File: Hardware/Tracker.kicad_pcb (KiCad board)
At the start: 2 copper layers, 233.7 x 114.2 mm, 58 parts, among them J1 Battery, J10 132134, J11 SPI_Programming, J2 Motor, J3 Wind, J4 RX, J5 TX, J6 GND, J7 GND, J8 GND, J9 Haeder_LED, U1 L7805, U2 ATmega328P-P, U3 LM317_TO-220, U4 L298N, U5 74HC123, U6 LM358, U7 GK9501, Y1 16MHz

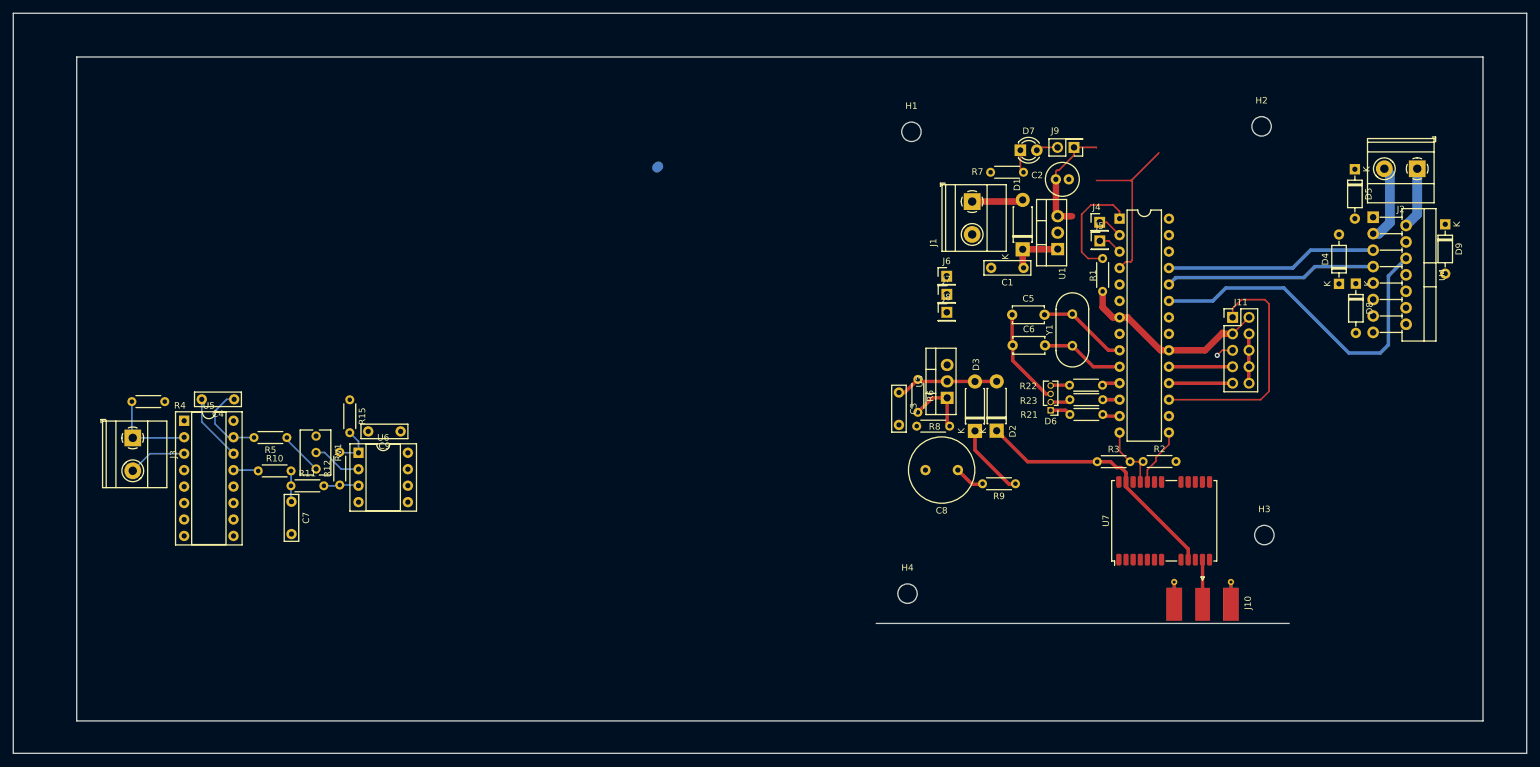
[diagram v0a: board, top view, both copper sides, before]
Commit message: Update of PCB
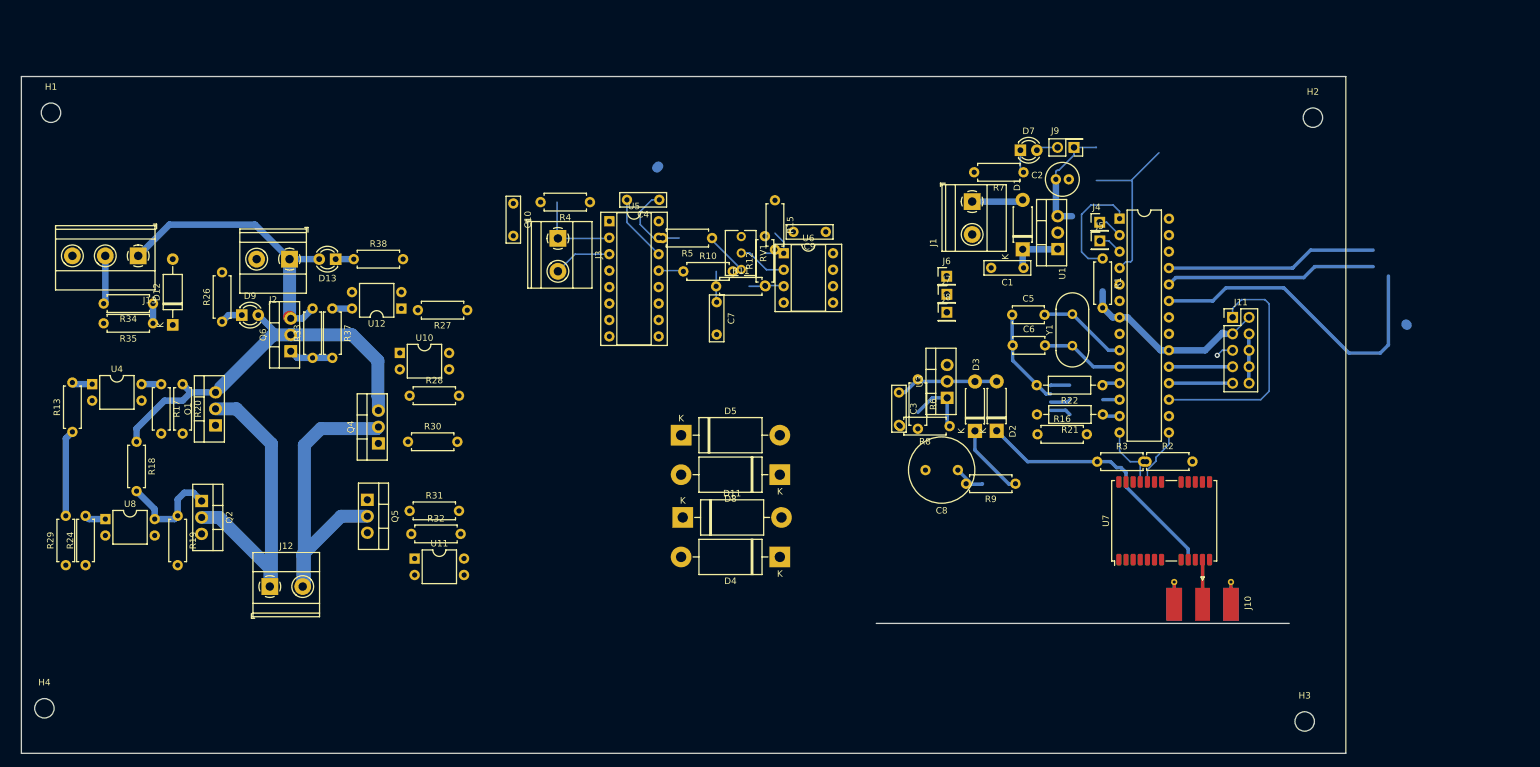
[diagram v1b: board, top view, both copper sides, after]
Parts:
- removed D6: LED_RBKG, Connector_PinHeader_1.27mm:PinHeader_1x04_P1.27mm_Vertical
- removed R23: 270, Resistor_THT:R_Axial_DIN0204_L3.6mm_D1.6mm_P5.08mm_Horizontal
- added C10: 100nF, Capacitor_THT:C_Rect_L7.0mm_W2.0mm_P5.00mm, F.Cu at (82.3, 68.1)
- added D11: 1N5406, Diode_THT:D_DO-201AD_P15.24mm_Horizontal, F.Cu at (108.5, 116.6)
- added D12: 3.3V, Diode_THT:D_A-405_P10.16mm_Horizontal, F.Cu at (29.7, 86.9)
- added D13: LED, LED_THT:LED_D3.0mm, F.Cu at (54.9, 76.7)
- added J12: Sortie Moteur, TerminalBlock_Phoenix:TerminalBlock_Phoenix_MKDS-1,5-2-5.08_1x02_P5.08mm_Horizontal, F.Cu at (44.7, 127.3)
- added J13: Position_Potentiometer, TerminalBlock_Phoenix:TerminalBlock_Phoenix_MKDS-1,5-3-5.08_1x03_P5.08mm_Horizontal, F.Cu at (24.4, 76.2)
- added Q1: IRF4905, Package_TO_SOT_THT:TO-220-3_Vertical, F.Cu at (36.3, 102.4)
- added Q2: IRF520, Package_TO_SOT_THT:TO-220-3_Vertical, F.Cu at (34.2, 114.0)
- added Q4: IRF4905, Package_TO_SOT_THT:TO-220-3_Vertical, F.Cu at (61.5, 105.2)
- added Q5: IRF520, Package_TO_SOT_THT:TO-220-3_Vertical, F.Cu at (59.8, 113.9)
- added Q6: IRF4905, Package_TO_SOT_THT:TO-220-3_Vertical, F.Cu at (47.9, 90.9)
- added R13: 470, Resistor_THT:R_Axial_DIN0207_L6.3mm_D2.5mm_P7.62mm_Horizontal, F.Cu at (14.2, 103.4)
- added R16: 470, Resistor_THT:R_Axial_DIN0207_L6.3mm_D2.5mm_P7.62mm_Horizontal, F.Cu at (163.2, 103.8)
- added R17: 2.2K, Resistor_THT:R_Axial_DIN0207_L6.3mm_D2.5mm_P7.62mm_Horizontal, F.Cu at (27.9, 96.0)
- added R18: 1K, Resistor_THT:R_Axial_DIN0207_L6.3mm_D2.5mm_P7.62mm_Horizontal, F.Cu at (24.1, 104.9)
- added R19: 100k, Resistor_THT:R_Axial_DIN0207_L6.3mm_D2.5mm_P7.62mm_Horizontal, F.Cu at (30.5, 116.3)
- added R20: 1K, Resistor_THT:R_Axial_DIN0207_L6.3mm_D2.5mm_P7.62mm_Horizontal, F.Cu at (31.2, 96.0)
- added R24: 470, Resistor_THT:R_Axial_DIN0207_L6.3mm_D2.5mm_P7.62mm_Horizontal, F.Cu at (16.3, 124.0)
- added R26: 3.3K, Resistor_THT:R_Axial_DIN0207_L6.3mm_D2.5mm_P7.62mm_Horizontal, F.Cu at (37.3, 86.4)
- added R27: 470, Resistor_THT:R_Axial_DIN0207_L6.3mm_D2.5mm_P7.62mm_Horizontal, F.Cu at (75.2, 84.6)
- added R28: 1K, Resistor_THT:R_Axial_DIN0207_L6.3mm_D2.5mm_P7.62mm_Horizontal, F.Cu at (66.3, 97.8)
- added R29: 470, Resistor_THT:R_Axial_DIN0207_L6.3mm_D2.5mm_P7.62mm_Horizontal, F.Cu at (13.2, 124.0)
- added R30: 2.2K, Resistor_THT:R_Axial_DIN0207_L6.3mm_D2.5mm_P7.62mm_Horizontal, F.Cu at (66.0, 104.9)
- added R31: 1K, Resistor_THT:R_Axial_DIN0207_L6.3mm_D2.5mm_P7.62mm_Horizontal, F.Cu at (66.3, 115.6)
- added R32: 100k, Resistor_THT:R_Axial_DIN0207_L6.3mm_D2.5mm_P7.62mm_Horizontal, F.Cu at (66.5, 119.1)
- added R33: 1k, Resistor_THT:R_Axial_DIN0207_L6.3mm_D2.5mm_P7.62mm_Horizontal, F.Cu at (51.3, 91.9)
- added R34: 2.7K, Resistor_THT:R_Axial_DIN0207_L6.3mm_D2.5mm_P7.62mm_Horizontal, F.Cu at (26.7, 83.6)
- added R35: 1K, Resistor_THT:R_Axial_DIN0207_L6.3mm_D2.5mm_P7.62mm_Horizontal, F.Cu at (26.7, 86.6)
- added R37: 2.2K, Resistor_THT:R_Axial_DIN0207_L6.3mm_D2.5mm_P7.62mm_Horizontal, F.Cu at (54.4, 84.3)
- added R38: 3.3K, Resistor_THT:R_Axial_DIN0207_L6.3mm_D2.5mm_P7.62mm_Horizontal, F.Cu at (57.7, 76.7)
- added U10: PC817, Package_DIP:DIP-4_W7.62mm, F.Cu at (64.8, 91.2)
- added U11: PC817, Package_DIP:DIP-4_W7.62mm, F.Cu at (67.1, 122.9)
- added U12: PC817, Package_DIP:DIP-4_W7.62mm, F.Cu at (65.0, 84.3)
- added U8: PC817, Package_DIP:DIP-4_W7.62mm, F.Cu at (19.3, 116.8)
- D2, D3: value D -> 1N4818
- D4, D5, D8: value 1N4148 -> 1N5406; footprint Diode_THT:D_DO-35_SOD27_P7.62mm_Horizontal -> Diode_THT:D_DO-201AD_P15.24mm_Horizontal
- D9: value 1N4148 -> LED; footprint Diode_THT:D_DO-35_SOD27_P7.62mm_Horizontal -> LED_THT:LED_D3.0mm
- J2: value Motor -> +24V
- R1, R10, R11, R12, R15, R2, R3, R4, R5, R6, R7, R8, R9: footprint Resistor_THT:R_Axial_DIN0204_L3.6mm_D1.6mm_P5.08mm_Horizontal -> Resistor_THT:R_Axial_DIN0207_L6.3mm_D2.5mm_P7.62mm_Horizontal
- R21, R22: footprint Resistor_THT:R_Axial_DIN0204_L3.6mm_D1.6mm_P5.08mm_Horizontal -> Resistor_THT:R_Axial_DIN0207_L6.3mm_D2.5mm_P10.16mm_Horizontal
- U4: value L298N -> PC817; footprint Package_TO_SOT_THT:TO-220-15_P2.54x2.54mm_StaggerOdd_Lead4.58mm_Vertical -> Package_DIP:DIP-4_W7.62mm
- moved U4 199.4 mm to (17.3, 96.0), turned to 0 degrees
- moved D9 186.3 mm to (40.4, 85.3), turned to 0 degrees
- moved J2 174.7 mm to (47.8, 76.7)
- moved H4 134.4 mm to (9.91, 146.1)
- moved H1 132.9 mm to (10.9, 54.1)
- moved D5 111.8 mm to (108.2, 103.9), turned to 0 degrees
- moved D4 96.1 mm to (123.4, 122.7), turned to 180 degrees
- moved D8 93.7 mm to (123.4, 110.0), turned to 180 degrees
- moved C4 72.5 mm to (104.8, 67.5)
- moved C7 72.5 mm to (113.7, 83.3)
- moved J3 72.5 mm to (89.2, 73.5)
- moved R10 72.5 mm to (108.5, 78.6)
- moved R11 72.5 mm to (113.6, 80.9)
- moved R12 72.5 mm to (121.1, 80.8)
- moved R15 72.5 mm to (122.7, 67.6)
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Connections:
- net /XTAL1 renamed /Crystal/XTAl_1
- net /XTAL2 renamed /Crystal/XTAl_2
- D4 pad 1: +BATT -> Net-(D4-K)
- D4 pad 2: Net-(D4-A) -> GND
- D5 pad 1: Net-(D4-A) -> +VCC_Motor
- D5 pad 2: GND -> Net-(D4-K)
- D8 pad 1: +BATT -> Net-(D11-A)
- D8 pad 2: Net-(D8-A) -> GND
- D9 pad 1: Net-(D8-A) -> Net-(D9-K)
- D9 pad 2: GND -> +VCC_Motor
- J2 pad 1: Net-(D8-A) -> +24V
- J2 pad 2: Net-(D4-A) -> GND
- U2 pad 11: Net-(U2-PD5) -> unconnected-(U2-PD5-Pad11)
- U2 pad 12: Net-(U2-PD6) -> unconnected-(U2-PD6-Pad12)
- U2 pad 13: Net-(U2-PD7) -> unconnected-(U2-PD7-Pad13)
- U2 pad 14: /GNSS/RX -> /GNSS/PPS
- U2 pad 15: /GNSS/TX -> /GNSS/RX
- U2 pad 16: /GNSS/PPS -> /GNSS/TX
- U2 pad 23: /Motors/EN_MOTOR -> /Motors/IN_B
- U2 pad 24: /Motors/IN2_MOTOR -> /Motors/IN_A
- U2 pad 25: /Motors/IN1_MOTOR -> /Motors/ENABLE
- U2 pad 26: unconnected-(U2-PC3-Pad26) -> /Motors/Pot_Measure
- U4 pad 1: GND -> Net-(R13-Pad2)
- U4 pad 2: Net-(D8-A) -> GND
- U4 pad 3: Net-(D4-A) -> GND
- U4 pad 4: +5V -> Net-(R17-Pad1)
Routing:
- net +VCC_Motor: track 0.00 -> 62.7 mm
- net /Motors/EN_MOTOR: track 53.9 -> 0.00 mm
- net /Motors/IN_B: track 0.00 -> 53.3 mm
- net Net-(D11-A): track 0.00 -> 51.9 mm
- net Net-(D4-K): track 0.00 -> 49.6 mm
- net /Motors/IN_A: track 0.00 -> 46.0 mm
- net +24V: track 0.00 -> 45.4 mm
- net /Motors/IN1_MOTOR: track 32.7 -> 0.00 mm
- net /Motors/ENABLE: track 0.00 -> 32.7 mm
- net /Motors/IN2_MOTOR: track 32.7 -> 0.00 mm
- net (no net): track 0.00 -> 18.8 mm
- net Net-(Q2-G): track 0.00 -> 16.4 mm
- net GND: track 31.7 -> 16.7 mm
- net Net-(D4-A): track 12.3 -> 0.00 mm
- net Net-(D8-A): track 9.48 -> 0.00 mm
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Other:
- board size 233.7 x 114.2 mm -> 204.5 x 104.5 mm
